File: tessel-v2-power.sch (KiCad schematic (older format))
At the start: 56 parts, among them J301 CONN_01X02, Q301 MMSS8550, U301 AAT4610, U302 AAT4610, U303 AP3417C, U304 AP3417C, U305 AP3418

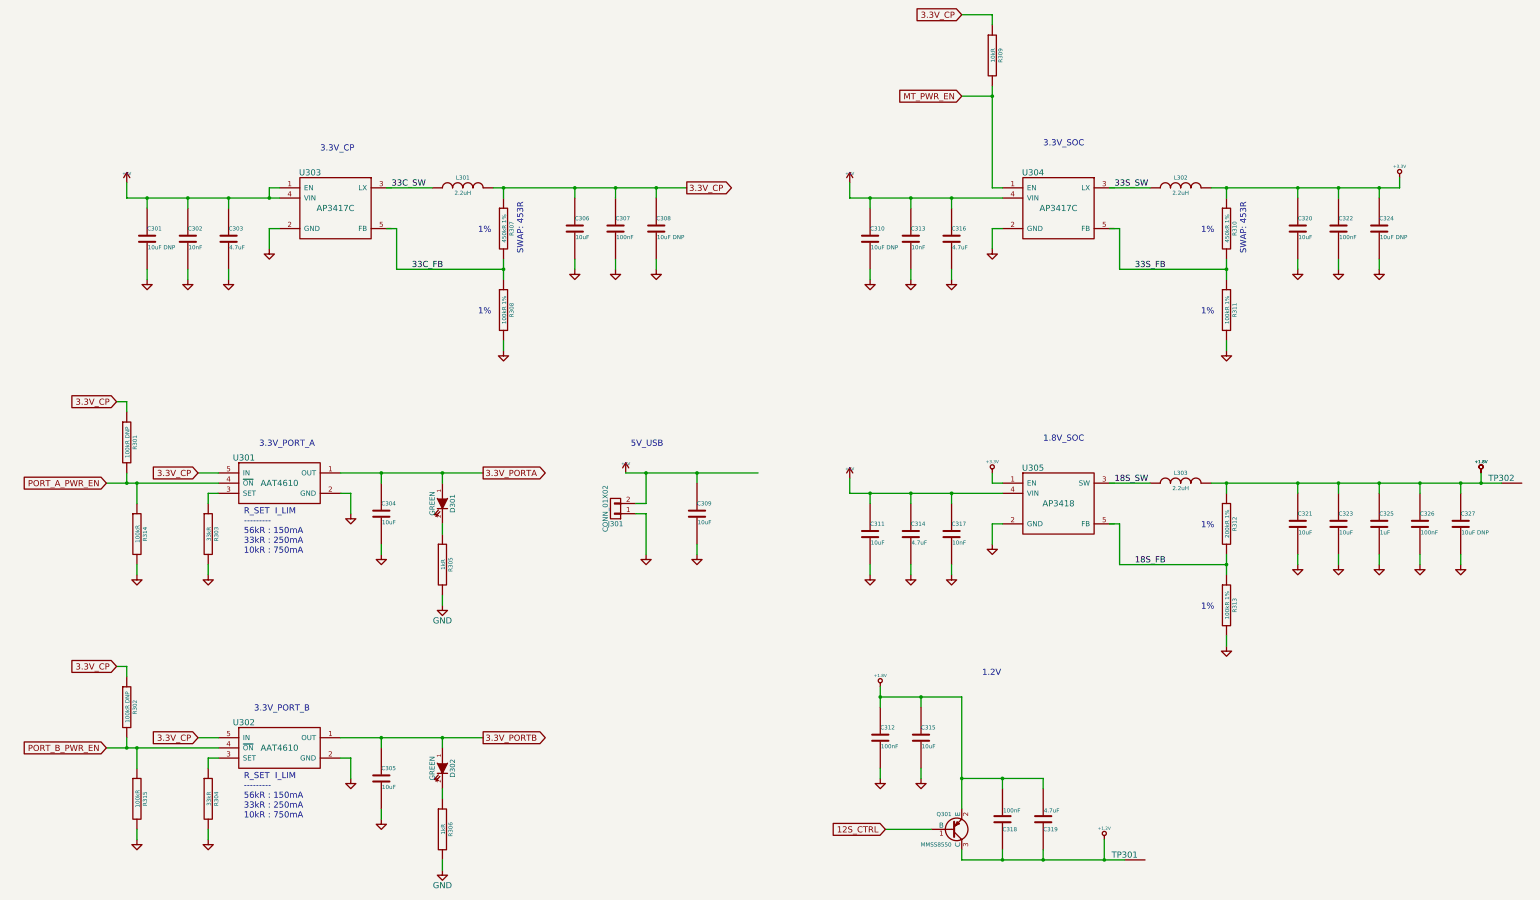
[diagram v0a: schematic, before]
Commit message: netlist, etc.
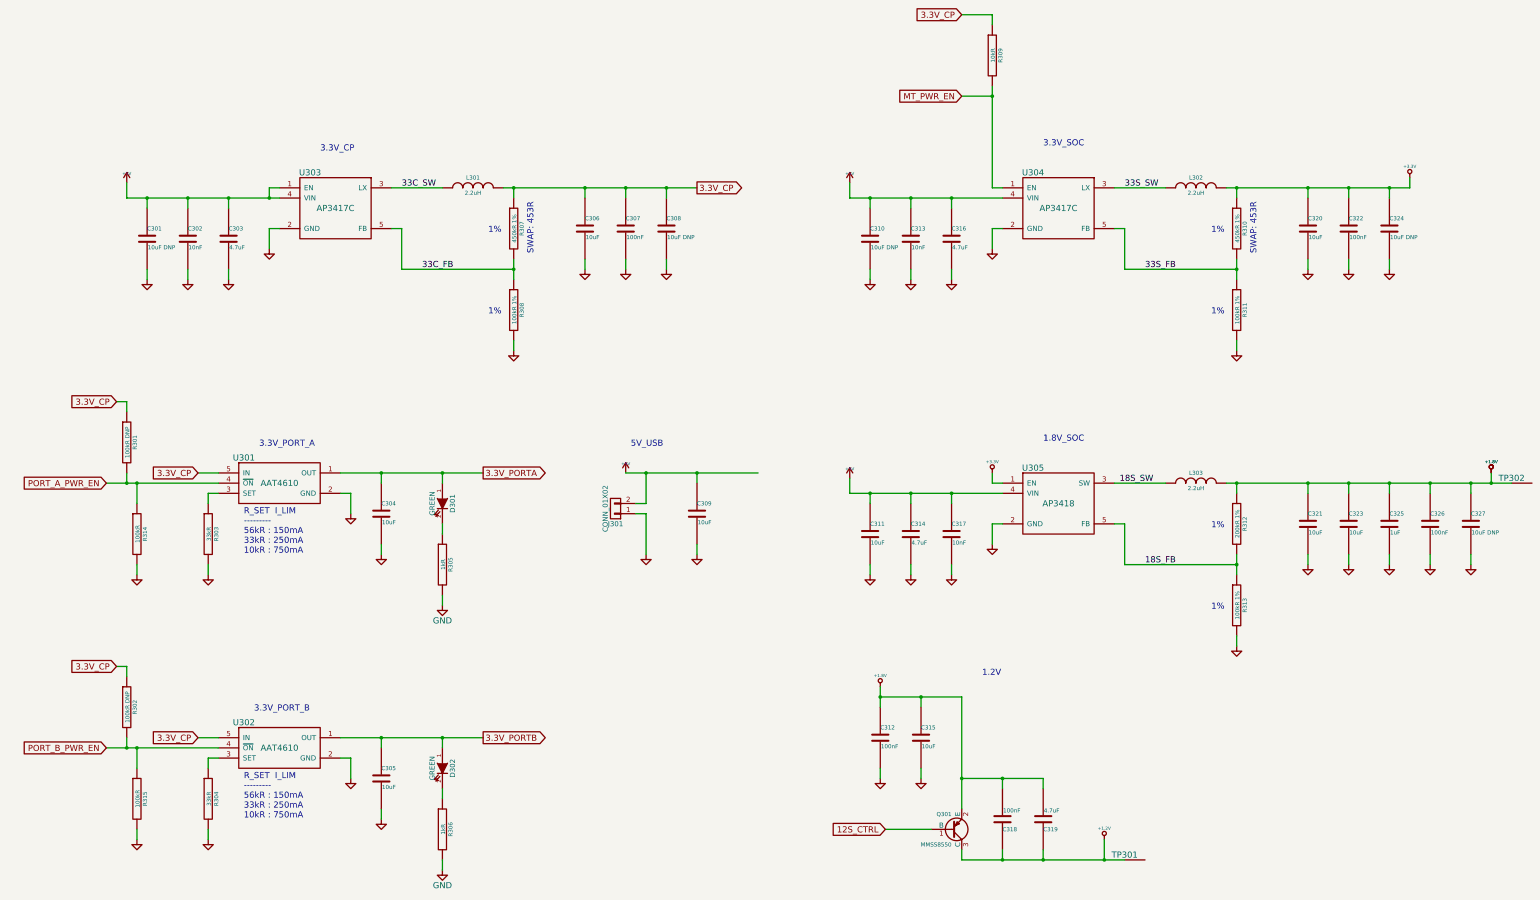
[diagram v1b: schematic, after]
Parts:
- J301: footprint (none) -> Pin_Headers:Pin_Header_Straight_1x02
- TP301, TP302: footprint (none) -> tm-kicad-lib:Testpoint
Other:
- moved on the sheet: C306, C307, C308, C320, C321, C322, C323, C324, C325, C326, C327, L301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
